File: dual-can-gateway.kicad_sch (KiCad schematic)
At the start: 86 parts, among them J3 Conn_01x02_Pin, Q1 AO3401A, Q2 2N7002, U1 STM32F446RETx, U2 STM32F446RETx, U3 ESP32-WROOM-32UE, U4 TJA1044GT-3, U5 TJA1044GT-3, U6 TJA1055T, U7 TJA1055T, U8 LM2596S-5, U9 AMS1117-3.3

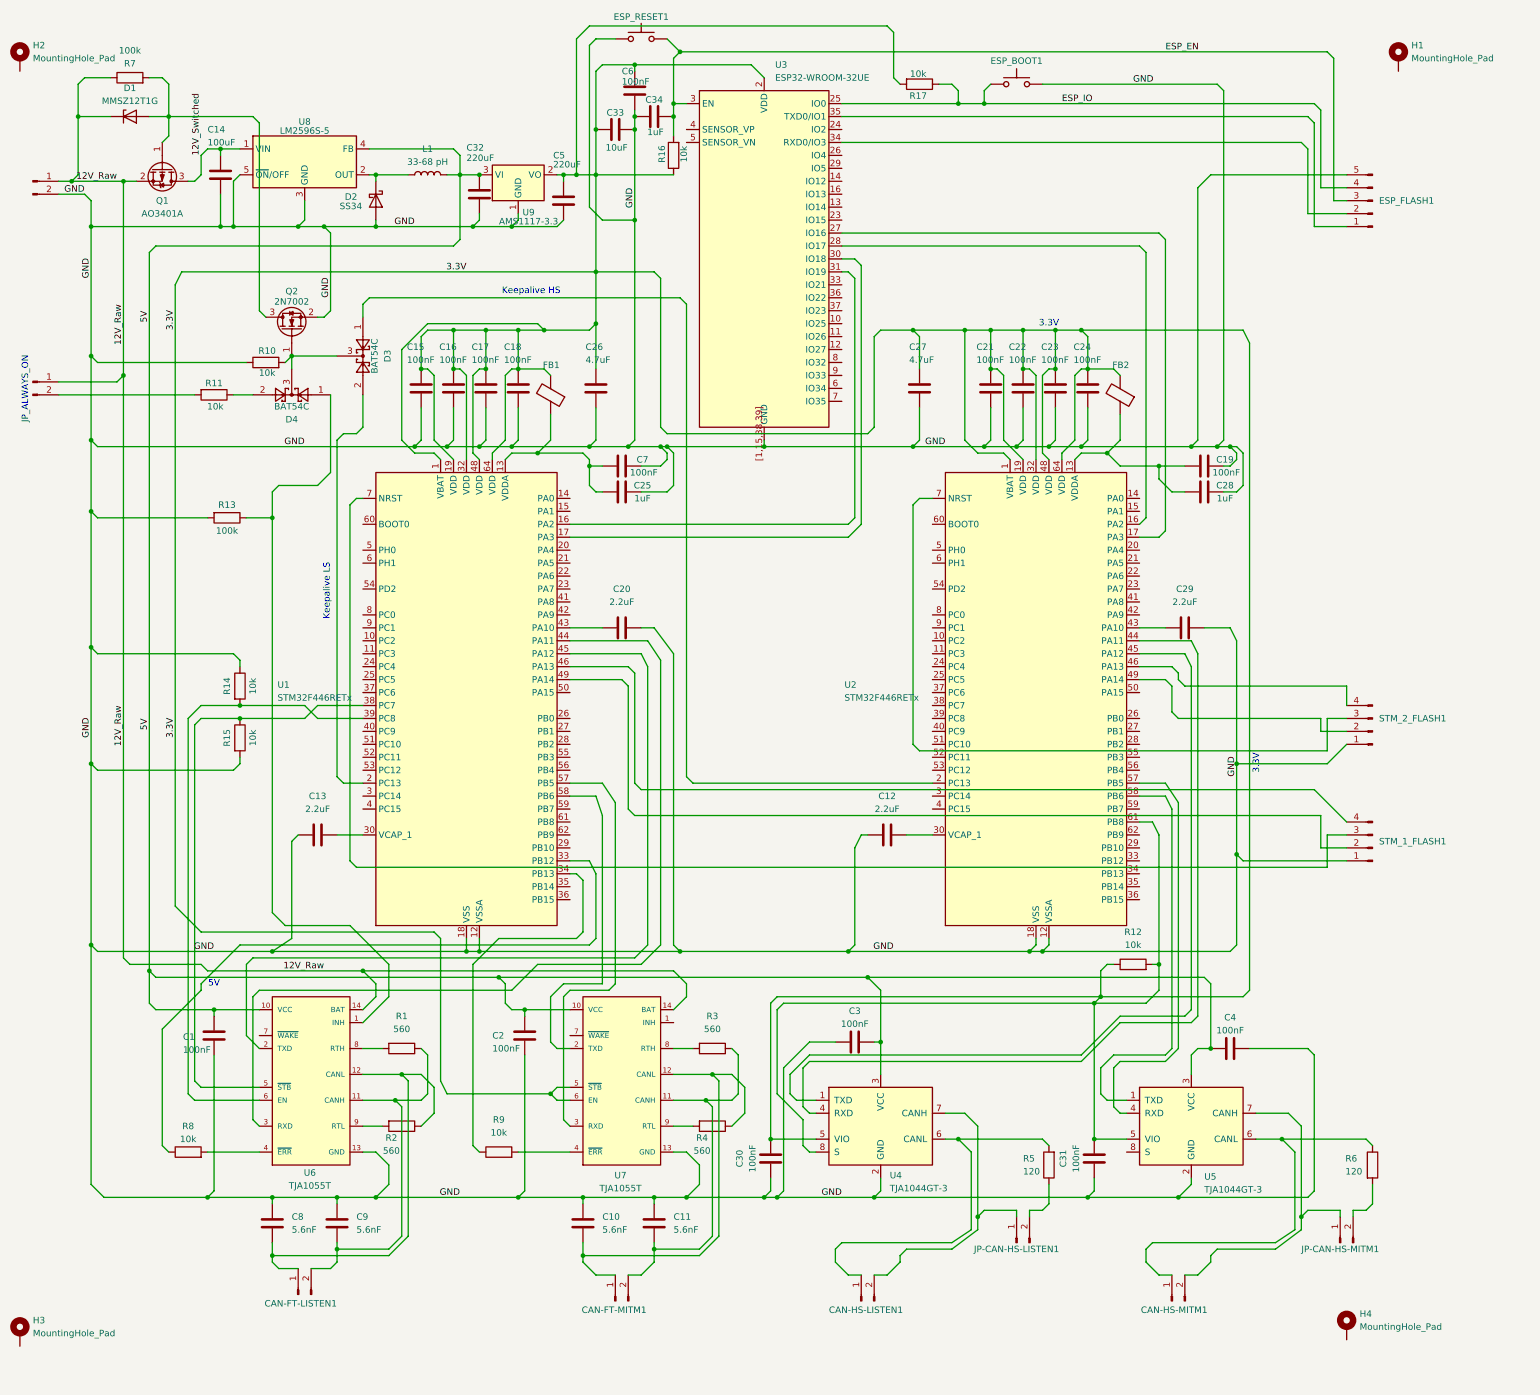
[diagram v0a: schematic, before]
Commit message: we're getting there
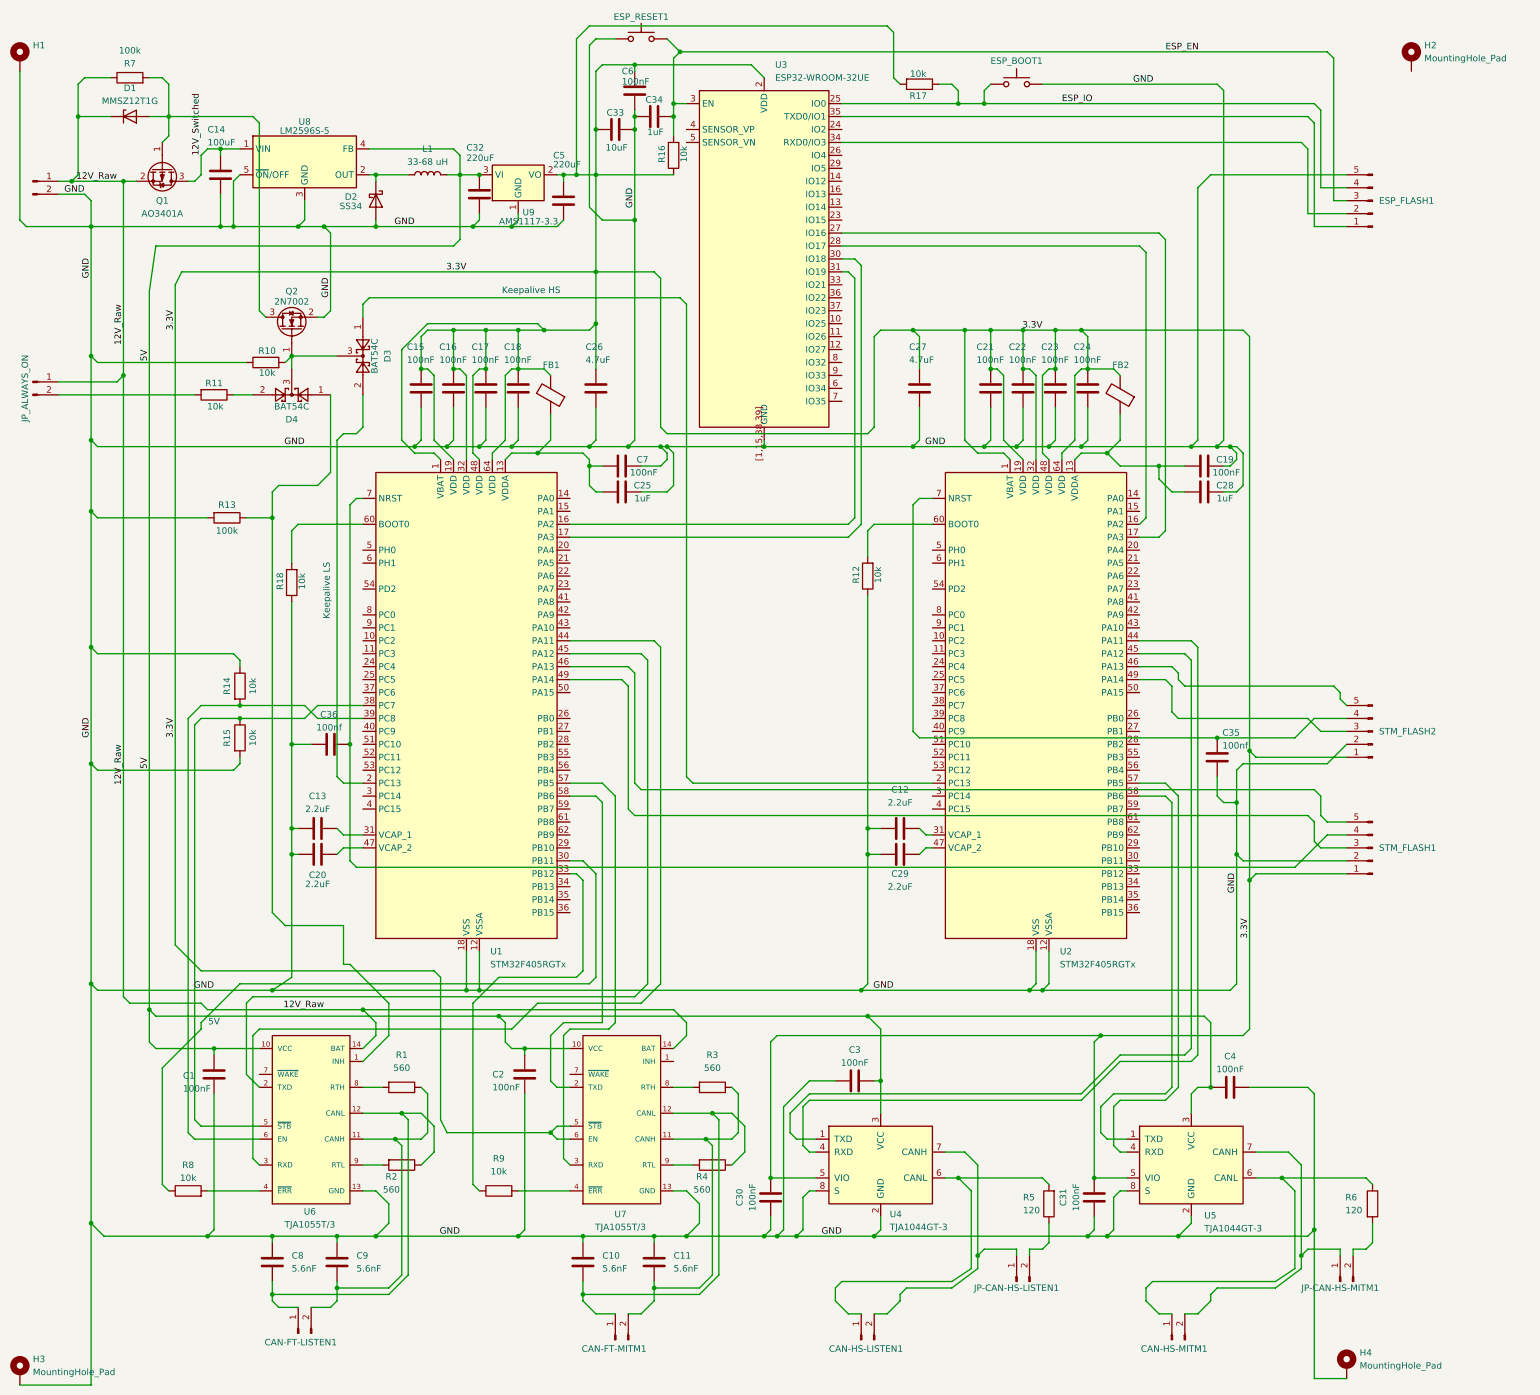
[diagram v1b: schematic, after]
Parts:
- removed STM_1_FLASH1, STM_2_FLASH1: Conn_01x04_Pin, Connector_PinHeader_2.54mm:PinHeader_1x04_P2.54mm_Vertical, symbol Connector:Conn_01x04_Pin
- removed U1, U2: STM32F446RETx, Package_QFP:LQFP-64_10x10mm_P0.5mm, symbol MCU_ST_STM32F4:STM32F446RETx
- added C35, C36: 100nf, Capacitor_SMD:C_0805_2012Metric, symbol Device:C
- added R18: 10k, Resistor_SMD:R_0805_2012Metric, symbol Device:R
- added STM_FLASH1, STM_FLASH2: Conn_01x05_Pin, Connector_PinHeader_2.54mm:PinHeader_1x05_P2.54mm_Vertical, symbol Connector:Conn_01x05_Pin
- added U1, U2: STM32F405RGTx, Package_QFP:LQFP-64_10x10mm_P0.5mm, symbol MCU_ST_STM32F4:STM32F405RGTx
- L1: value 33-68 pH -> 33-68 uH
- U6, U7: value TJA1055T -> TJA1055T/3
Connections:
- net 3.3V: now also STM_FLASH1.1 (Pin_1), STM_FLASH2.1 (Pin_1), U1.1 (VBAT), U1.19 (VDD), U1.32 (VDD), U1.48 (VDD), U1.64 (VDD), U2.1 (VBAT), U2.19 (VDD), U2.32 (VDD), U2.48 (VDD), U2.64 (VDD); no longer R12.1, R12.2, U4.8 (S)
- net GND: now also C20.1, C29.1, H1.1, H3.1, H4.1, R12.1, U4.8 (S), U5.8 (S), C35.1, C36.2, R18.1, STM_FLASH1.2 (Pin_2), STM_FLASH2.2 (Pin_2), U1.12 (VSSA), U1.18 (VSS), U1.63 (VSS), U2.12 (VSSA), U2.18 (VSS), U2.63 (VSS); no longer C20.2, C29.2
- net at R9.1: now also U1.33 (PB12)
- net at U4.1 (TXD): now also U2.45 (PA12)
- net at U4.4 (RXD): now also U2.44 (PA11)
- net at C13.2: now also U1.31 (VCAP_1)
- net at D3.1: now also U2.2 (PC13)
- net at D3.2: now also U1.2 (PC13)
- net at R14.2, U6.6 (EN): now also U1.39 (PC8)
- net at C19.1, C28.1, FB2.1: now also U2.13 (VDDA)
- net at U3.28 (IO17): now also U2.16 (PA2)
- net at U3.27 (IO16): now also U2.17 (PA3)
- net at C12.2: now also U2.31 (VCAP_1)
- net at U5.4 (RXD): now also U2.57 (PB5)
- net at U5.1 (TXD): now also U2.58 (PB6)
- net at C25.1, C7.1, FB1.1: now also U1.13 (VDDA)
- net at U6.2 (TXD): now also U1.45 (PA12)
- net at U6.3 (RXD): now also U1.44 (PA11)
- net at R15.1, U6.5 (~{STB}): now also U1.38 (PC7)
- net at U7.2 (TXD): now also U1.58 (PB6)
- net at U7.3 (RXD): now also U1.57 (PB5)
- net at U3.30 (IO18): now also U1.17 (PA3)
- net at U3.31 (IO19): now also U1.16 (PA2)
- net at R8.1: now also U1.30 (PB11)
- new net: STM_FLASH1.3 (Pin_3), U1.49 (PA14)
- new net: C36.1, STM_FLASH1.4 (Pin_4), U1.7 (NRST)
- new net: STM_FLASH1.5 (Pin_5), U1.46 (PA13)
- new net: R12.2, U2.60 (BOOT0)
- new net: C29.2, U2.47 (VCAP_2)
- new net: C35.2, STM_FLASH2.4 (Pin_4), U2.7 (NRST)
- new net: R18.2, U1.60 (BOOT0)
- new net: C20.2, U1.47 (VCAP_2)
- new net: STM_FLASH2.5 (Pin_5), U2.46 (PA13)
- new net: STM_FLASH2.3 (Pin_3), U2.49 (PA14)
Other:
- note removed: "3.3V"
- moved on the sheet: C1, C10, C11, C12, C13, C2, C20, C29, C3, C30, C31, C4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
